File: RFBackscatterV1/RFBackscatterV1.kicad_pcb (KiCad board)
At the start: 2 copper layers, 34.6 x 51.9 mm, 13 parts, among them J1 SMA-J-P-H-RA-TH1, U1 SIT1534AI-H4-DCC-00.001E, U3 74LVC1GU04DRL

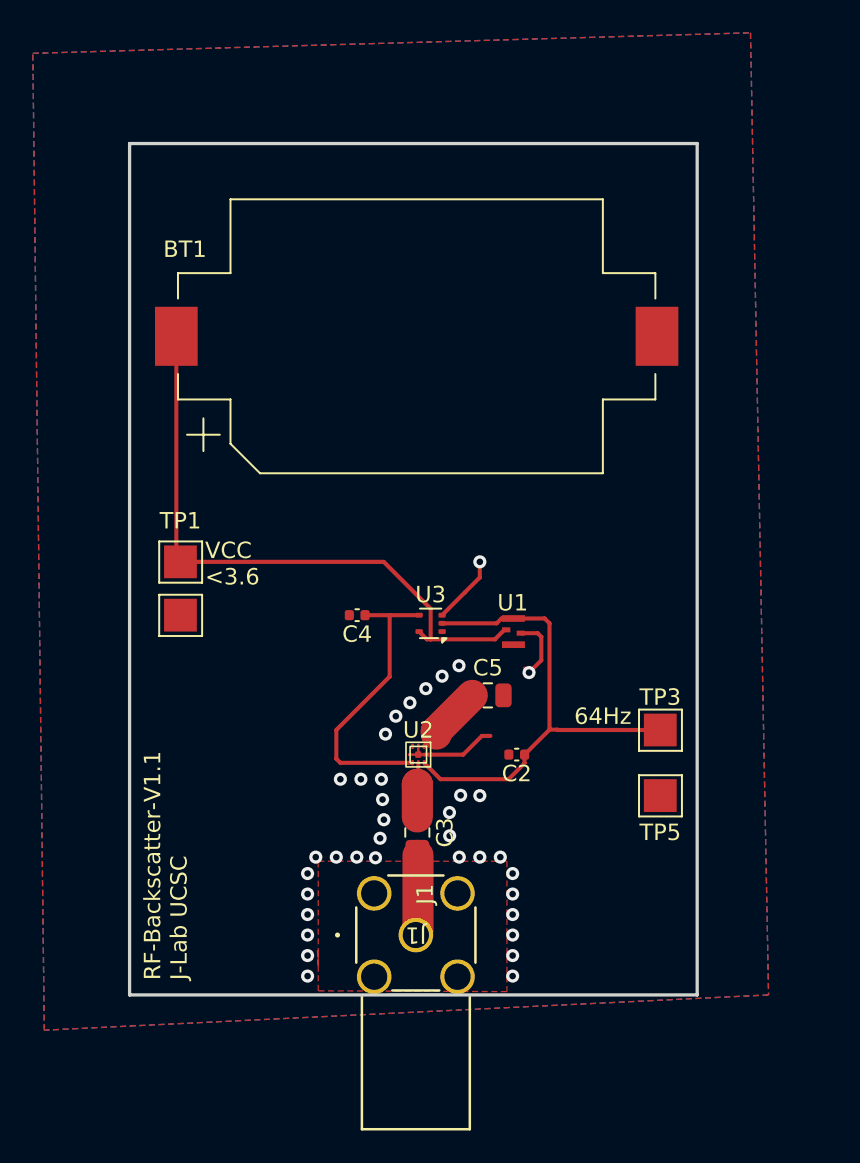
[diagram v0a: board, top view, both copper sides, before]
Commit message: JLPCB order
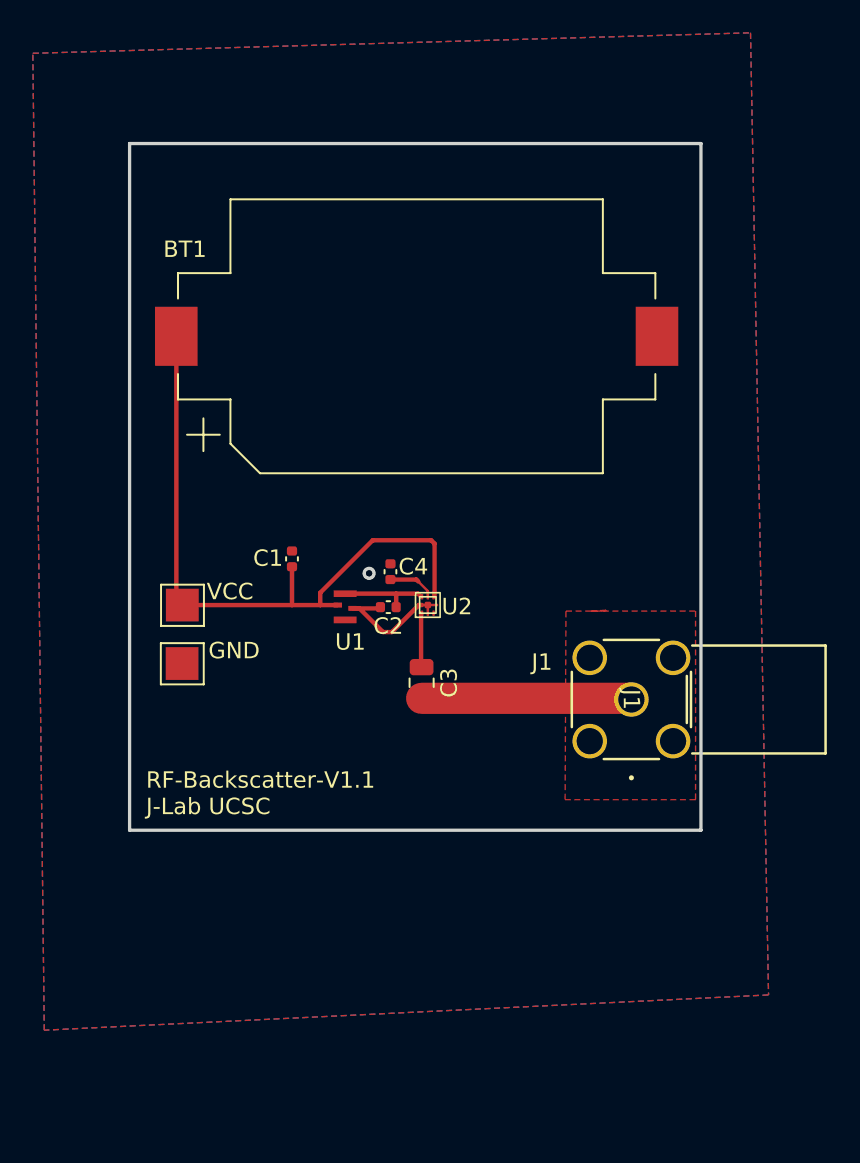
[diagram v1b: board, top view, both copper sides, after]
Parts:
- removed C5: 10nF, Capacitor_SMD:C_0805_2012Metric
- removed TP3: CLK_OUT, JLab_FP:EpicTestPointV1
- removed TP6: GND, JLab_FP:EpicTestPointV1
- removed U3: 74LVC1GU04DRL, Package_TO_SOT_SMD:SOT-553
- added C1: 33pF, Capacitor_SMD:C_0402_1005Metric, F.Cu at (156.3, 70.3)
- C3: value 10nF -> 100pF
- C4: value 33pF -> 100pF
- moved TP5 30.2 mm to (150.1, 79.4)
- moved J1 19.5 mm to (177.0, 78.9), turned to -90 degrees
- moved U2 12.8 mm to (159.8, 73.1), turned to 90 degrees
- moved C2 11.9 mm to (162.2, 73.3)
- moved U1 10.4 mm to (159.5, 73.2)
- moved C3 9.13 mm to (164.2, 77.9)
- moved C4 3.34 mm to (162.3, 71.1), turned to 90 degrees
- moved TP1 2.64 mm to (150.1, 75.9)
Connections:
- BT1 pad 1: 3V0 -> Net-(BT1-+)
- C3 pad 1: Net-(U2-INPUT) -> Net-(U2-OUTPUT1)
- C4 pad 1: Net-(U2-VCTL2) -> Net-(U2-INPUT)
- TP1 pad 1: 3V0 -> Net-(BT1-+)
- U1 pad 4: 3V0 -> Net-(BT1-+)
- U2 pad 3: Net-(U2-OUTPUT2) -> unconnected-(U2-OUTPUT2-Pad3)
- U2 pad 4: Net-(U2-VCTL2) -> Net-(BT1-+)
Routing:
- net Net-(BT1-+): track 0.00 -> 40.7 mm
- net 3V0: track 37.9 -> 0.00 mm
- net Net-(U1-CLK_Out): track 29.6 -> 5.53 mm
- net Net-(U2-VCTL2): track 18.1 -> 0.00 mm
- net Net-(C3-Pad2): track 5.30 -> 12.8 mm
- net GND: track 12.9 -> 7.26 mm, vias 37 -> 1
- net Net-(U2-OUTPUT1): track 4.26 -> 3.30 mm
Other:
- board size 34.6 x 51.9 mm -> 34.8 x 41.9 mm
- board text added: "GND"
- board text added: "VCC"
- board text removed: "64Hz"
- board text removed: "VCC <3.6"
